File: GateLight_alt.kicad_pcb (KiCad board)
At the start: 2 copper layers, 57.5 x 27.5 mm, 9 parts

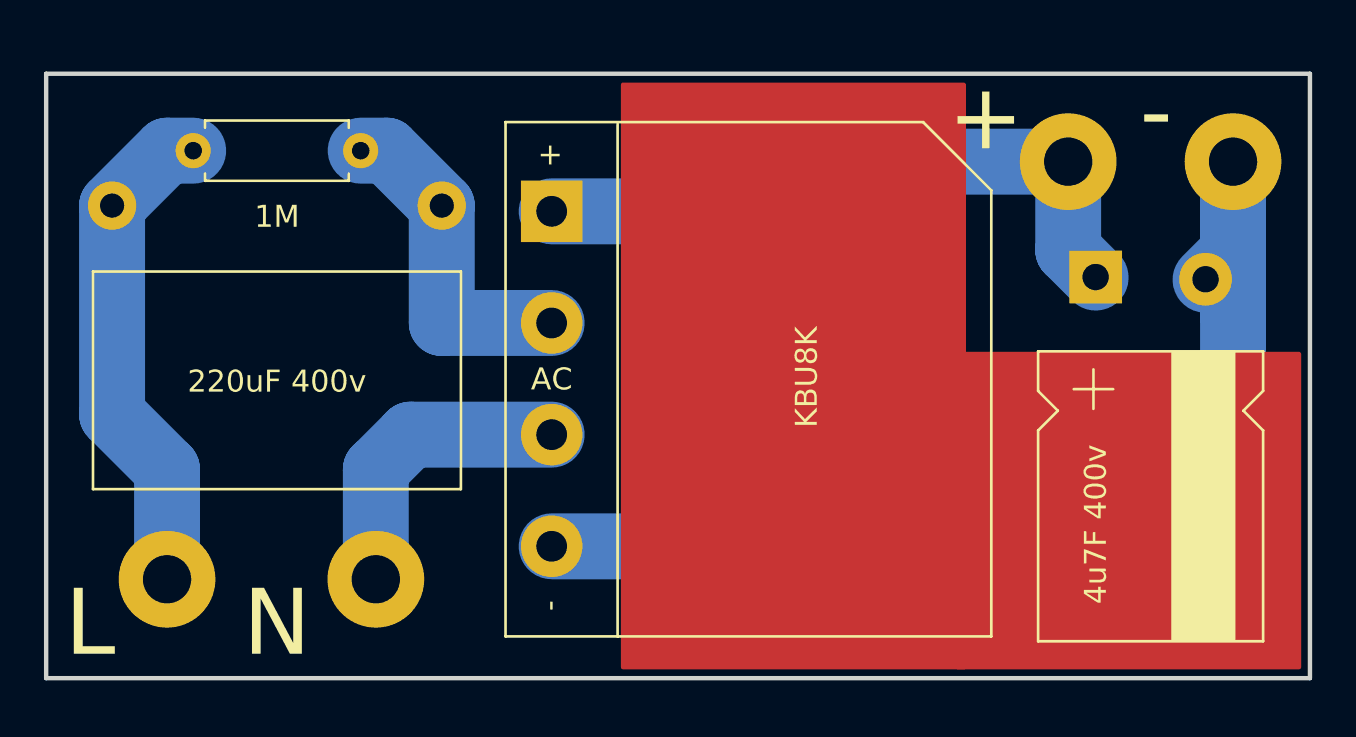
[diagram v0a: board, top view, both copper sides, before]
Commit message: first pass at fabrication; two designs
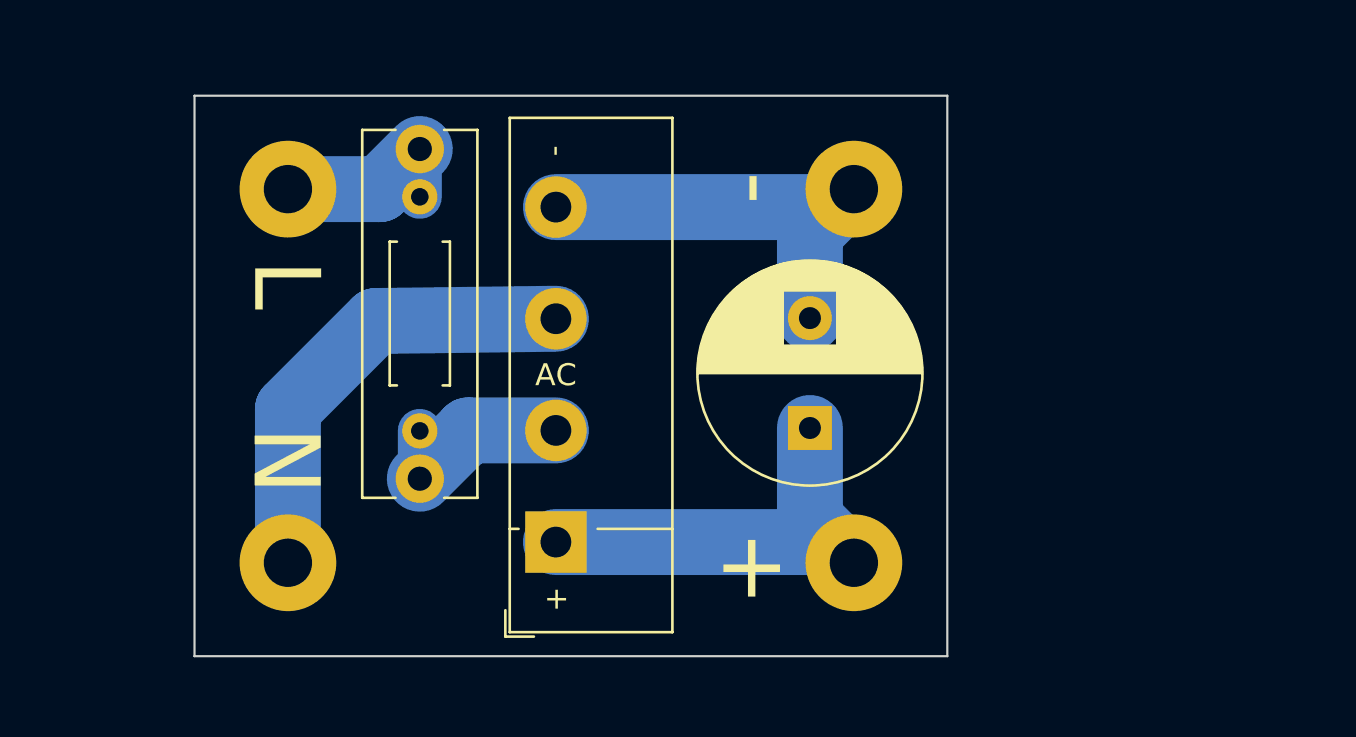
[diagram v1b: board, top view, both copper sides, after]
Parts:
- C101: footprint Capacitor_THT:C_Rect_L16.5mm_W9.2mm_P15.00mm_MKT -> Capacitor_THT:C_Rect_L16.5mm_W5.0mm_P15.00mm_MKT
- C102: value 4u7F 400v -> 4u7F; footprint 3805_Misc:CP_Radial_L13.0mm_D10.0mm_P5.00mm_Horizontal -> Capacitor_THT:CP_Radial_D10.0mm_P5.00mm
- moved H103 20.7 mm to (109.2, 99.2)
- moved Ge 19.0 mm to (101.4, 90.6)
- moved H101 18.6 mm to (83.5, 82.2)
- moved C102 17.7 mm to (107.2, 93.1)
- moved H104 17.3 mm to (109.2, 82.2)
- moved C101 12.5 mm to (89.5, 95.4), turned to 90 degrees
- moved R101 10.9 mm to (89.5, 84.1), turned to -90 degrees
- moved H102 4.07 mm to (83.5, 99.2)
- moved D101 0.27 mm to (95.7, 98.3)
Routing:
- net Net-(C102-Pad2): track 55.3 -> 20.6 mm
- net Net-(C101-Pad2): track 22.8 -> 8.93 mm
- net Net-(C102-Pad1): track 30.2 -> 20.9 mm
- net Net-(D101-Pad3): track 13.7 -> 20.8 mm
- net Net-(C101-Pad1): track 15.1 -> 9.28 mm
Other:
- board size 57.5 x 27.5 mm -> 34.2 x 25.5 mm
- board text added: "Edd Inglis, December 2023"
- board text removed: "Edd Inglis December 2023"
